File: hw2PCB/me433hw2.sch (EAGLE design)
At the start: 20 parts, among them J1 USB-MB-H

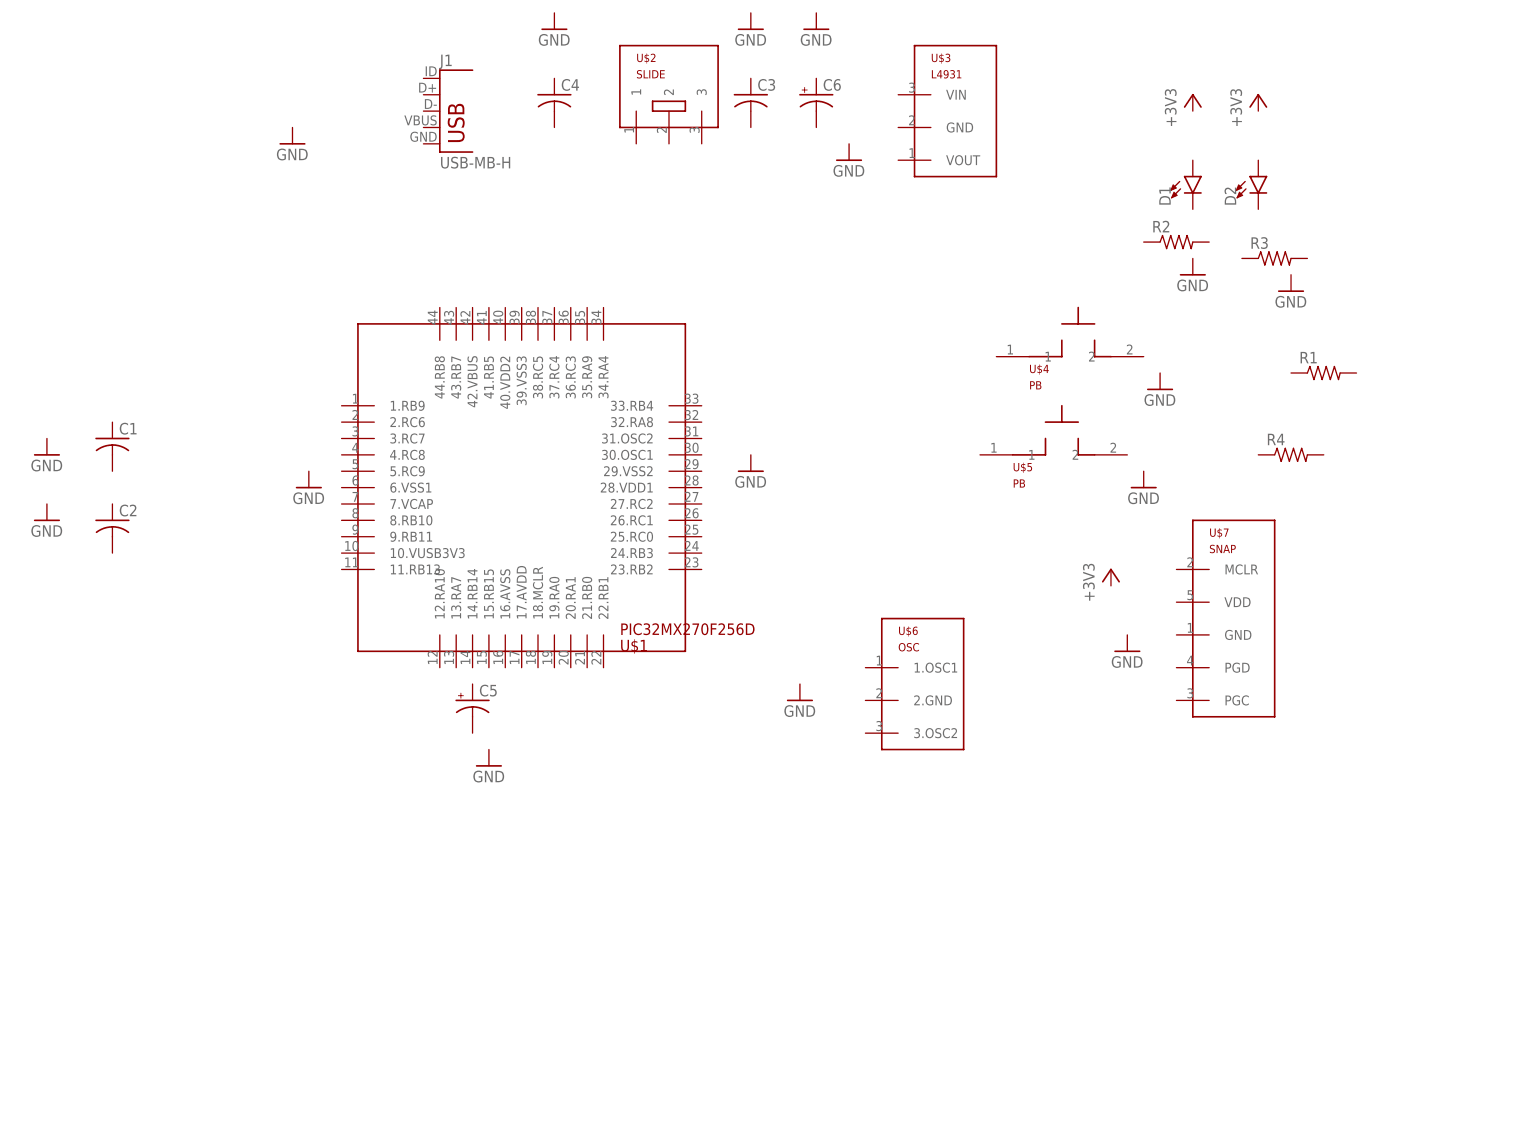
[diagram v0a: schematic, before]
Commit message: Fixed hw2 update
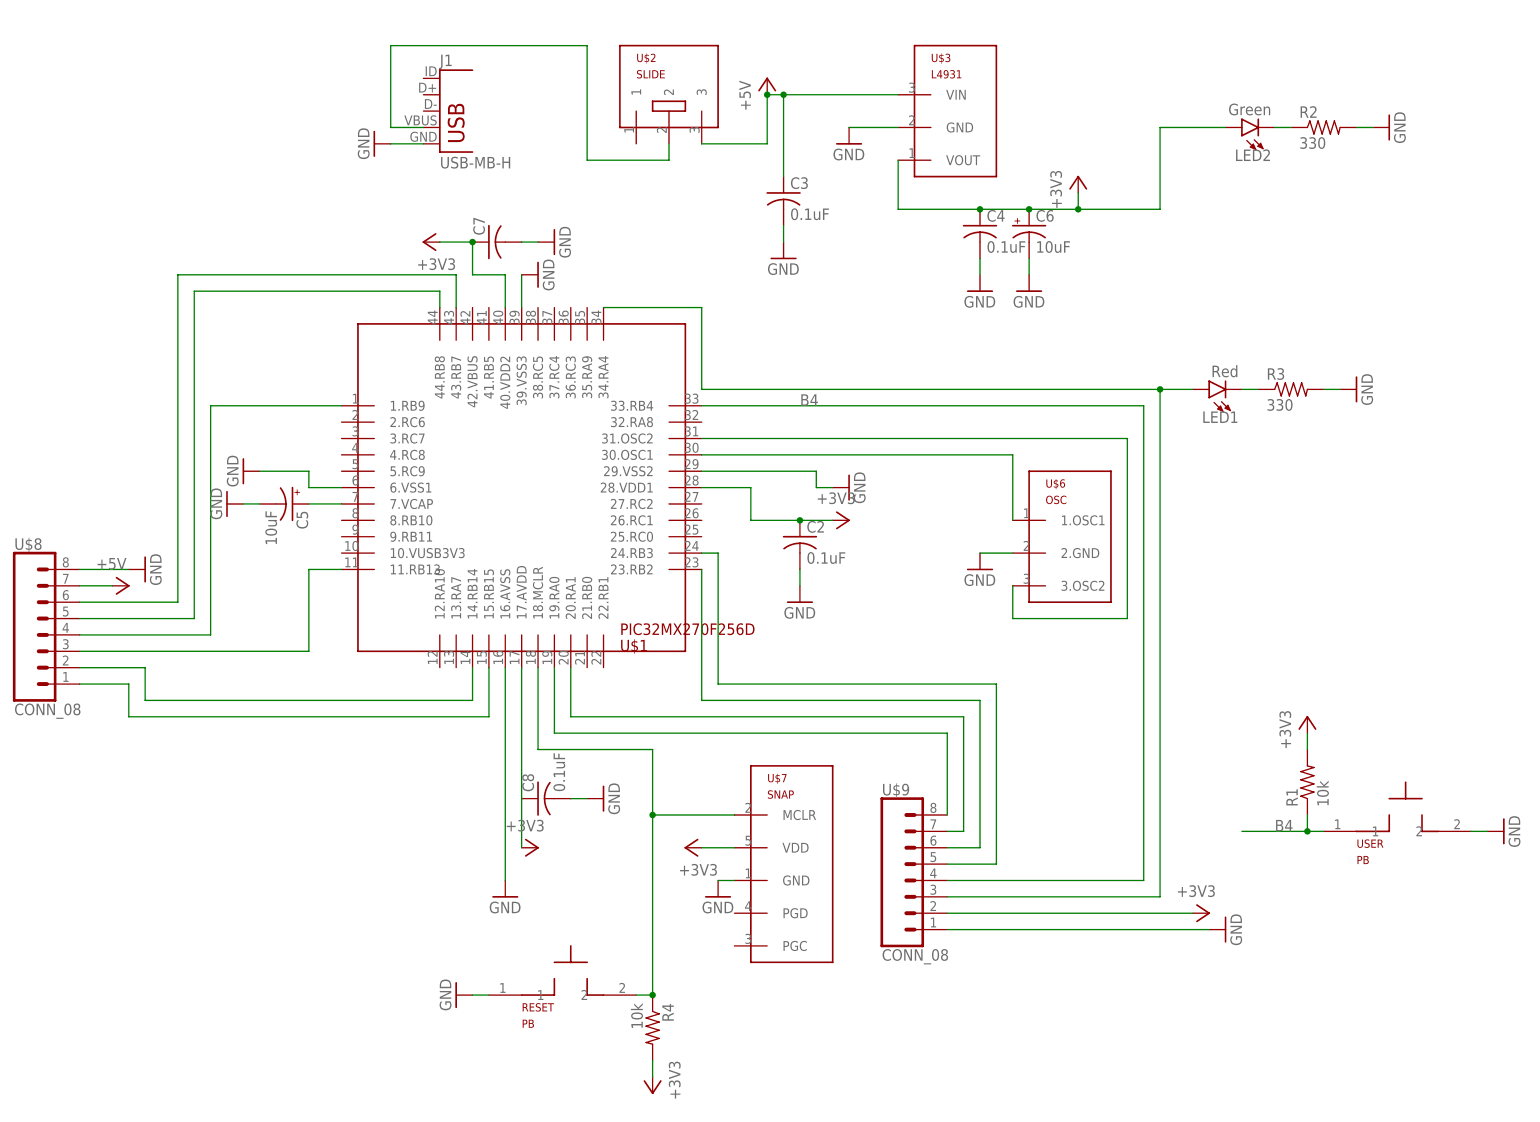
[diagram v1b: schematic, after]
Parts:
- removed C1: (no value), me433hw2:C-US025-025X050
- removed D1, D2: (no value), me433hw2:LED3MM
- removed U$4, U$5: PB, me433hw2:PB
- added C7: (no value), me433hw2:C-US025-025X050
- added C8: 0.1uF, me433hw2:C-US025-025X050
- added LED1: Red, me433hw2:LED3MM
- added LED2: Green, me433hw2:LED3MM
- added RESET, USER: PB, me433hw2:PB
- added U$8, U$9: CONN_08, me433hw2:CONN_08
- C2, C3, C4: value (none) -> 0.1uF
- C5, C6: value (none) -> 10uF
- R1, R4: value (none) -> 10k
- R2, R3: value (none) -> 330
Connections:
- new net +3V3: C2.1, C4.1, C6.+, C7.1, LED2.A, R1.2, R4.2, U$1.28.VDD1, U$1.40.VDD2, U$3.VOUT, U$7.VDD, U$9.2
- new net +5V: C3.1, U$2.3, U$3.VIN, U$8.7
- new net B4: R1.1, U$1.33.RB4, U$9.4, USER.1
- new net GND: C2.2, C3.2, C4.2, C5.-, C6.-, C7.2, C8.2, J1.GND, R2.2, R3.2, RESET.1, U$1.16.AVSS, U$1.29.VSS2, U$1.39.VSS3, U$1.6.VSS1, U$3.GND, U$6.2.GND, U$7.GND, U$8.8, U$9.1, USER.2
- new net N$1: U$1.31.OSC2, U$6.3.OSC2
- new net N$10: U$1.20.RA1, U$9.7
- new net N$11: U$1.23.RB2, U$9.6
- new net N$12: U$1.24.RB3, U$9.5
- new net N$14: LED1.A, U$1.34.RA4, U$9.3
- new net N$15: U$1.43.RB7, U$8.6
- new net N$16: U$1.44.RB8, U$8.5
- new net N$17: U$1.1.RB9, U$8.4
- new net N$18: U$1.11.RB13, U$8.3
- new net N$19: U$1.14.RB14, U$8.2
- new net N$2: U$1.30.OSC1, U$6.1.OSC1
- new net N$20: U$1.15.RB15, U$8.1
- new net N$3: J1.VBUS, U$2.2
- new net N$4: R4.1, RESET.2, U$1.18.MCLR, U$7.MCLR
- new net N$5: LED2.C, R2.1
- new net N$6: LED1.C, R3.1
- new net N$7: C5.+, U$1.7.VCAP
- new net N$8: C8.1, U$1.17.AVDD
- new net N$9: U$1.19.RA0, U$9.8
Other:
- moved on the sheet: C2, C3, C4, C5, C6, R1, R2, R3, R4, U$6, U$7
